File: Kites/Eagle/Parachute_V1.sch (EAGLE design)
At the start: 24 parts, among them Q1 MOSFET-NCH, Q2 MOSFET-NCH, U1 ITSYBITSY_5V, X1 MSTBA8

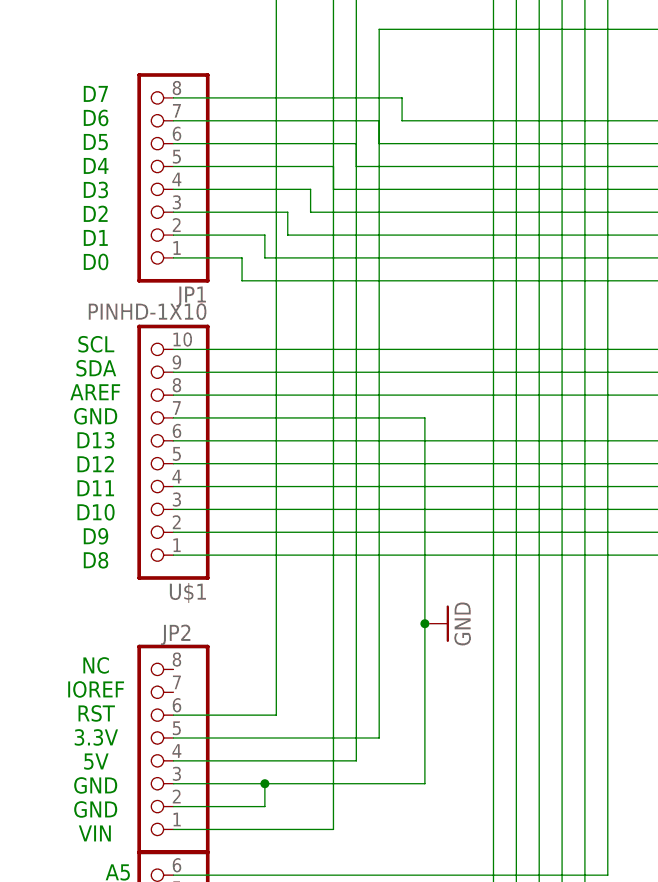
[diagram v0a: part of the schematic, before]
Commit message: Updated repository to match most recent revisions
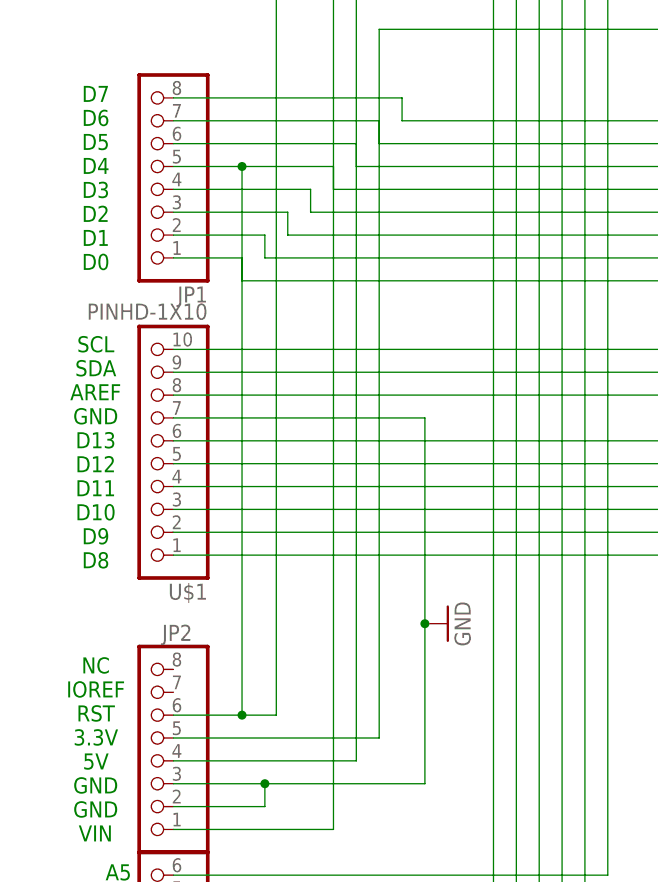
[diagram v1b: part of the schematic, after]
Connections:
- removed net N$23: JP2.6, U1.RST
- net N$22: now also JP2.6, U1.RST
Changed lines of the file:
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@@
 <wire x1="35.56" y1="111.76" x2="35.56" y2="114.3" width="0.1524" layer="91"/>
 <pinref part="JP1" gate="G$1" pin="5"/>
-<wire x1="35.56" y1="114.3" x2="17.78" y2="114.3" width="0.1524" layer="91"/>
+<wire x1="35.56" y1="114.3" x2="25.4" y2="114.3" width="0.1524" layer="91"/>
+<pinref part="U1" gate="G$1" pin="RST"/>
+<wire x1="25.4" y1="114.3" x2="17.78" y2="114.3" width="0.1524" layer="91"/>
+<wire x1="81.28" y1="162.56" x2="73.66" y2="162.56" width="0.1524" layer="91"/>
+<wire x1="73.66" y1="162.56" x2="73.66" y2="165.1" width="0.1524" layer="91"/>
+<wire x1="73.66" y1="165.1" x2="63.5" y2="165.1" width="0.1524" layer="91"/>
+<wire x1="63.5" y1="165.1" x2="63.5" y2="162.56" width="0.1524" layer="91"/>
+<wire x1="63.5" y1="162.56" x2="29.21" y2="162.56" width="0.1524" layer="91"/>
+<wire x1="29.21" y1="162.56" x2="29.21" y2="53.34" width="0.1524" layer="91"/>
+<pinref part="JP2" gate="G$1" pin="6"/>
+<wire x1="29.21" y1="53.34" x2="25.4" y2="53.34" width="0.1524" layer="91"/>
+<wire x1="25.4" y1="53.34" x2="17.78" y2="53.34" width="0.1524" layer="91"/>
+<wire x1="25.4" y1="114.3" x2="25.4" y2="53.34" width="0.1524" layer="91"/>
+<junction x="25.4" y="114.3"/>
+<junction x="25.4" y="53.34"/>
 </segment>
 </net>
@@
 </segment>
 </net>
-<net name="N$23" class="0">
-<segment>
-<pinref part="U1" gate="G$1" pin="RST"/>
-<wire x1="81.28" y1="162.56" x2="73.66" y2="162.56" width="0.1524" layer="91"/>
-<wire x1="73.66" y1="162.56" x2="73.66" y2="165.1" width="0.1524" layer="91"/>
-<wire x1="73.66" y1="165.1" x2="63.5" y2="165.1" width="0.1524" layer="91"/>
-<wire x1="63.5" y1="165.1" x2="63.5" y2="162.56" width="0.1524" layer="91"/>
-<wire x1="63.5" y1="162.56" x2="29.21" y2="162.56" width="0.1524" layer="91"/>
-<wire x1="29.21" y1="162.56" x2="29.21" y2="53.34" width="0.1524" layer="91"/>
-<pinref part="JP2" gate="G$1" pin="6"/>
-<wire x1="29.21" y1="53.34" x2="17.78" y2="53.34" width="0.1524" layer="91"/>
-</segment>
-</net>
